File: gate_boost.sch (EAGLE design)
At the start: 57 parts, among them IC1 LM324D, IC2 SP34063A_BOOST_REG

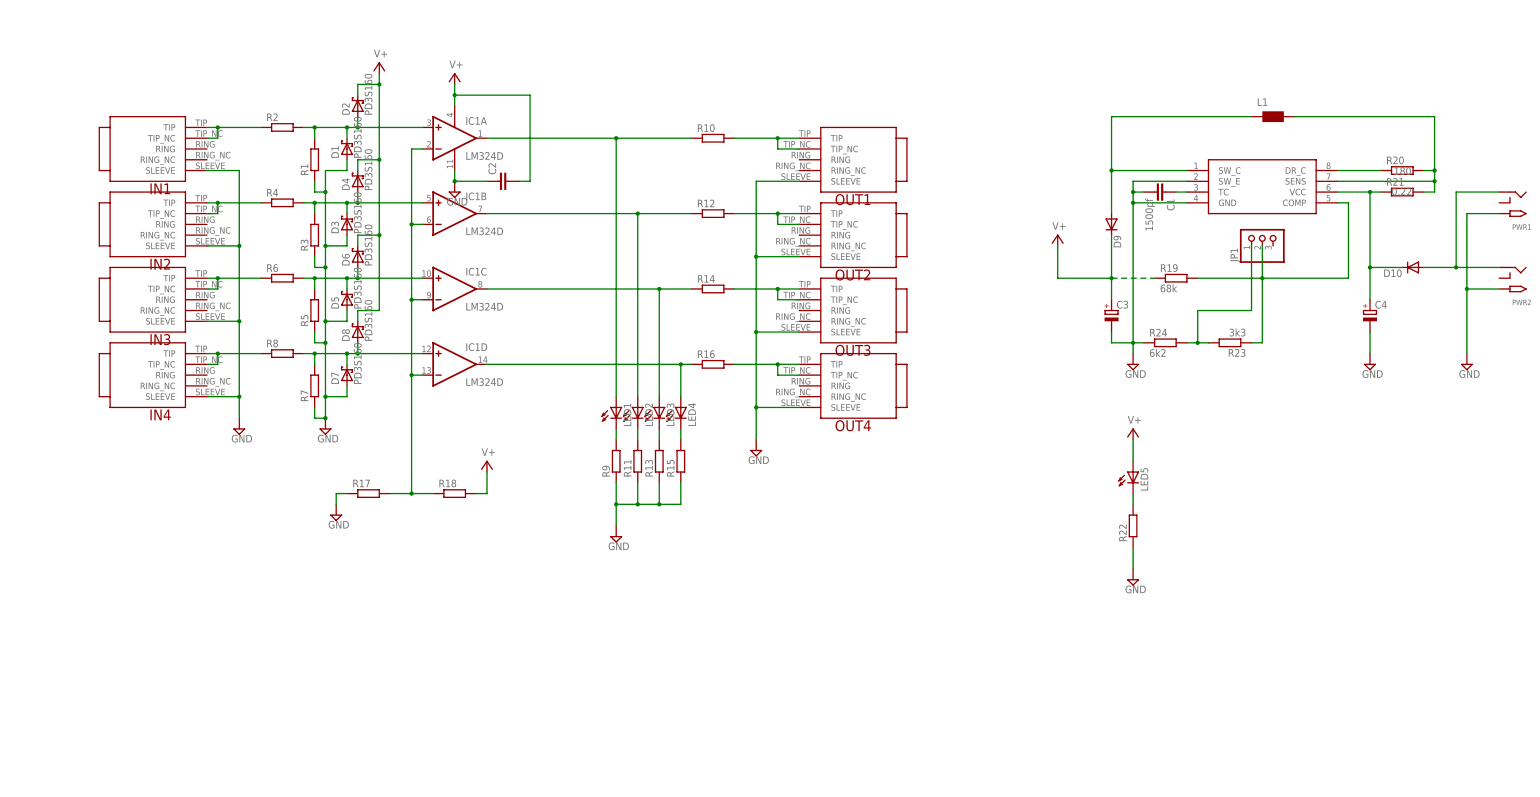
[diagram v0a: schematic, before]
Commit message: charge pump
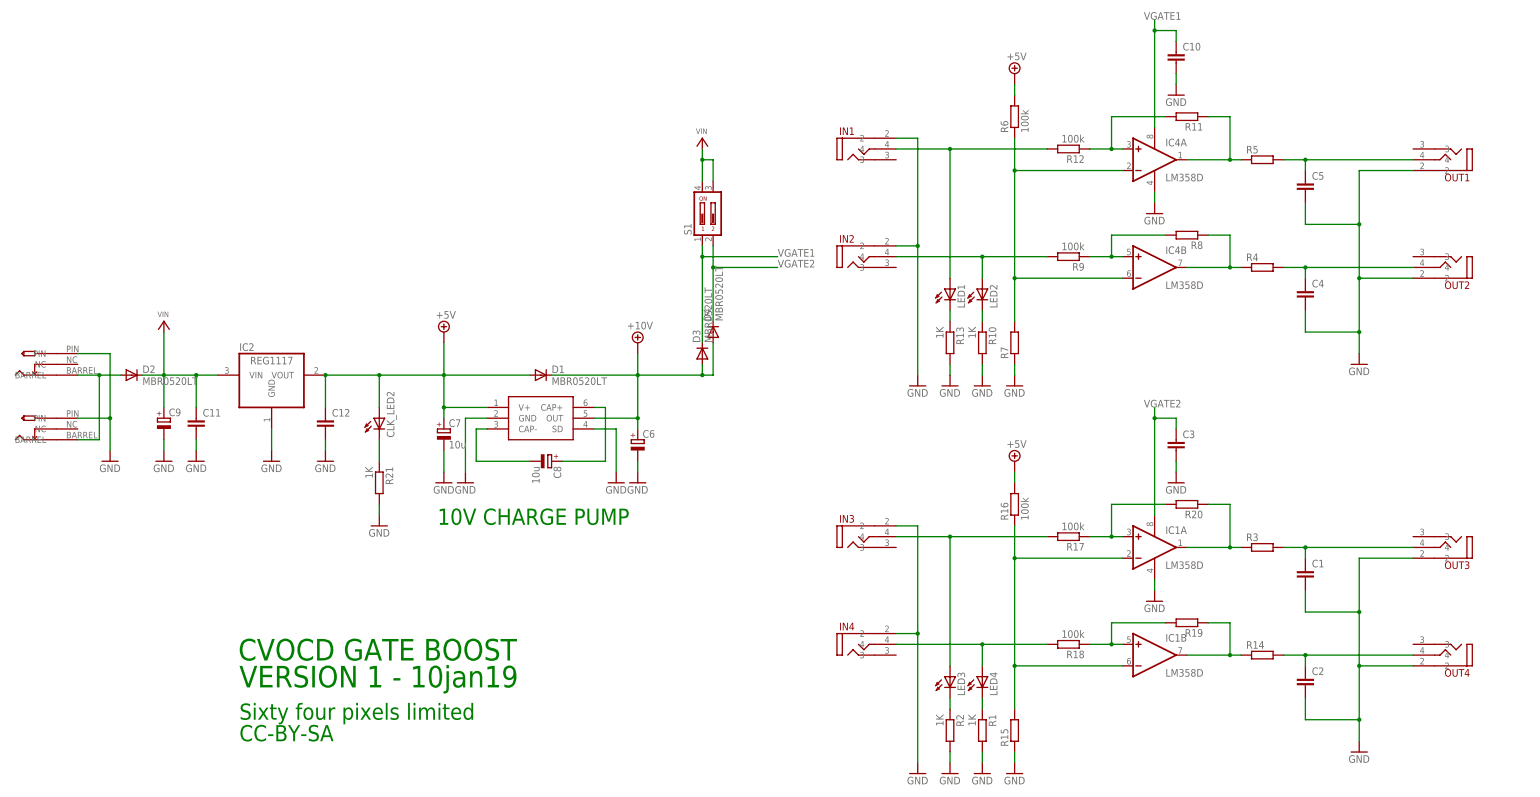
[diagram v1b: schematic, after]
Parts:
- removed D10, D9: CGRM4001-G, diode:CGRM4001-G
- removed D5, D6, D7, D8: PD3S160, diode:PD3S160
- removed JP1: (no value), pinhead:PINHD-1X3
- removed L1: (no value), wuerth-elektronik:WE-PD_S/M
- removed LED5: (no value), adafruit:LED3MM
- removed PWR1, PWR2: 2.1MMJACKTHM, adafruit:2.1MMJACKTHM
- removed R22: (no value), rcl:R-EU_R0805
- removed R23: 3k3, rcl:R-EU_R0805
- removed R24: 6k2, rcl:R-EU_R0805
- added C10, C11, C12, C5: (no value), resistor:C-EUC0805
- added C6: (no value), rcl:CPOL-EUSMCA
- added C7, C8: 10u, rcl:CPOL-EUSMCA
- added C9: (no value), rcl:CPOL-EUE2-5
- added CLK_LED2: (no value), led:LED3MM
- added IC3: LM27675M5_CHARGEPUMP, jason_eagle6:LM27675M5_CHARGEPUMP
- added IC4: LM358D, linear:LM358D
- added S1: (no value), switch-dil:DIP02YL
- added U$1, U$2: PWR_SOCKET_2_1MM, jason_eagle6:PWR_SOCKET_2_1MM
- C1: value 1500pf -> (none); device rcl:C-EUC0805 -> resistor:C-EUC0805
- C2: device rcl:C-EUC0805 -> resistor:C-EUC0805
- C3, C4: device rcl:CPOL-EUE2.5-6 -> resistor:C-EUC0805
- D1, D2, D3, D4: value PD3S160 -> MBR0520LT; device diode:PD3S160 -> diode:MBR0520LT
- IC1: value LM324D -> LM358D; device linear:LM324D -> linear:LM358D
- IC2: value SP34063A_BOOST_REG -> REG1117; device jason_eagle6:SP34063A_BOOST_REG -> burr-brown:REG1117
- IN1, IN2, IN3, IN4, OUT1, OUT2, OUT3, OUT4: value TRUCONNECTJACK -> VERTICAL_3_5MM_SOCKET; device jason_eagle6:TRUCONNECTJACK -> jason_eagle6:VERTICAL_3_5MM_SOCKET
- LED1, LED2, LED3, LED4: device adafruit:LED3MM -> led:LED3MM
- R1, R10, R13, R2: value (none) -> 1K
- R12, R16, R17, R18, R6, R9: value (none) -> 100k
- R19: value 68k -> (none)
- R20: value 180 -> (none)
- R21: value 0.22 -> 1K
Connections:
- removed net N$18: IC1C.OUT, LED3.A, R14.1
- removed net N$22: IC2.DR_C, R20.1
- removed net N$24: C4.+, D10.C, IC2.VCC, R21.1
- removed net N$25: D10.A, PWR1.RING, PWR2.RING
- removed net N$27: LED1.C, R9.2
- removed net N$30: LED2.C, R11.2
- removed net N$31: LED3.C, R13.2
- removed net N$32: LED4.C, R15.2
- removed net N$34: LED5.C, R22.2
- removed net N$6: D5.C, D6.A, IC1C.+IN, R5.2, R6.2
- removed net V+: C2.2, C3.+, D2.C, D4.C, D6.C, D8.C, D9.C, IC1P.V+, LED5.A, R18.2, R19.1
- new net +10V: C6.+, D1.C, D3.A, D4.A, IC3.OUT
- new net +5V: C12.1, C7.+, CLK_LED2.A, D1.A, IC2.VOUT, IC3.V+, R16.2, R6.2
- new net IN1: IN1.4, LED1.A, R12.2
- new net IN2: IN2.4, LED2.A, R9.2
- new net IN3: IN3.4, LED3.A, R17.2
- new net IN4: IN4.4, LED4.A, R18.2
- new net N$38: C8.+, IC3.CAP+
- new net N$39: C8.-, IC3.CAP-
- new net VGATE1: C10.1, D3.C, IC4P.V+, S1.1
- new net VGATE2: C3.1, D4.C, IC1P.V+, S1.2
- new net VIN: C11.1, C9.+, D2.C, IC2.VIN, S1.3, S1.4
- net GND: now also C10.2, C11.2, C12.2, C2.2, C3.2, C4.2, C5.2, C6.-, C7.-, C9.-, IC3.GND, IC3.SD, IC4P.V-, IN1.2, IN2.2, IN3.2, IN4.2, OUT1.2, OUT2.2, OUT3.2, OUT4.2, R1.2, R10.2, R13.2, R2.2, R21.2, U$1.PIN, U$2.PIN; no longer C2.1, C3.-, C4.-, D1.A, D3.A, D5.A, D7.A, IC2.SW_E, IN1.SLEEVE, IN2.SLEEVE, IN3.SLEEVE, IN4.SLEEVE, OUT1.SLEEVE, OUT2.SLEEVE, OUT3.SLEEVE, OUT4.SLEEVE, PWR1.TIP, PWR2.TIP, R1.1, R11.1, R13.1, R17.1, R22.1, R24.1, R3.1, R5.1, R9.1
- net N$1: now also IC4A.-IN, IC4B.-IN, R6.1, R7.2; no longer IN1.TIP, IN1.TIP_NC, R2.1
- net N$10: now also IC1B.OUT, R14.1, R19.1; no longer IC1A.-IN, IC1B.-IN, IC1C.-IN, IC1D.-IN, R17.2, R18.1
- net N$11: now also IC1A.OUT, R20.1, R3.1; no longer OUT1.TIP, OUT1.TIP_NC, R10.2
- net N$12: now also IC4B.OUT, R4.1, R8.1; no longer OUT2.TIP, OUT2.TIP_NC, R12.2
- net N$13: now also IC1A.-IN, IC1B.-IN, R15.2, R16.1; no longer OUT3.TIP, OUT3.TIP_NC, R14.2
- net N$14: now also LED3.C, R2.1; no longer OUT4.TIP, OUT4.TIP_NC, R16.2
- net N$15: now also LED4.C, R1.1; no longer C1.1, IC2.TC
- net N$16: now also IC1A.+IN, R17.1, R20.2; no longer D9.A, IC2.SW_C, L1.1
- net N$17: now also IC1B.+IN, R18.1, R19.2; no longer IC1B.OUT, LED2.A, R12.1
- net N$19: now also C5.1, OUT1.4, R5.2; no longer IC1D.OUT, LED4.A, R16.1
- net N$2: now also LED1.C, R13.1; no longer IN2.TIP, IN2.TIP_NC, R4.1
- net N$20: now also C4.1, OUT2.4, R4.2; no longer IC2.COMP, JP1.2, R19.2, R23.1
- net N$21: now also D2.A, U$1.BARREL, U$2.BARREL; no longer JP1.1, R23.2, R24.2
- net N$23: now also CLK_LED2.C, R21.1; no longer IC2.SENS, L1.2, R20.2, R21.2
- net N$3: now also LED2.C, R10.1; no longer IN3.TIP, IN3.TIP_NC, R6.1
- net N$4: now also IC4A.+IN, R11.2, R12.1; no longer IN4.TIP, IN4.TIP_NC, R8.1
- net N$5: now also IC4B.+IN, R9.1; no longer D7.C, D8.A, IC1D.+IN, R7.2
- net N$7: now also C1.1, OUT3.4; no longer D3.C, D4.A, IC1B.+IN, R4.2
- net N$8: now also C2.1, OUT4.4, R14.2; no longer D1.C, D2.A, IC1A.+IN, R1.2, R2.2
- net N$9: now also IC4A.OUT, R11.1, R5.1; no longer IC1A.OUT, LED1.A, R10.1
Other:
- note added: "10V CHARGE PUMP"
- note added: "CC-BY-SA"
- note added: "CVOCD GATE BOOST"
- note added: "Sixty four pixels limited"
- note added: "VERSION 1 - 10jan19"
- moved on the sheet: C1, C2, IC1A, IC1B, LED1, LED2, LED3, LED4, R1, R10, R11, R12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
